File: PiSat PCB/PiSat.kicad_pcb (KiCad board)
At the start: 4 copper layers, 85 x 56 mm, 125 parts, among them IC1 PNT-SG3FS-TR, J1 Conn_01x05_Pin, J3 Conn_01x06_Pin, J4 Conn_01x03_Pin, J5 Conn_01x05_Pin, J6 Conn_01x05_Pin, Q7 AO3407A, SW1 MSK12C02, SW2 SKRPACE010, SW3 SKRPACE010, U1 BQ24075RGTR, U12 AP2112K-3.3, U4 DW03C_C41367942, U5 SMA-KWE_C7498154, U6 ESP32-C3-MINI-1U-N4, X1 X322512MSB4SI

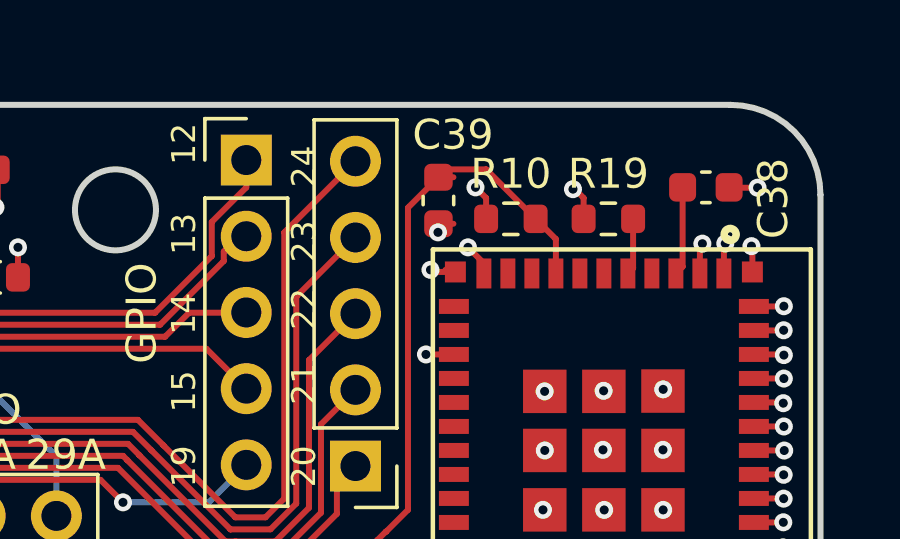
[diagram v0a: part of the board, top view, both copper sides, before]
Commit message: sync
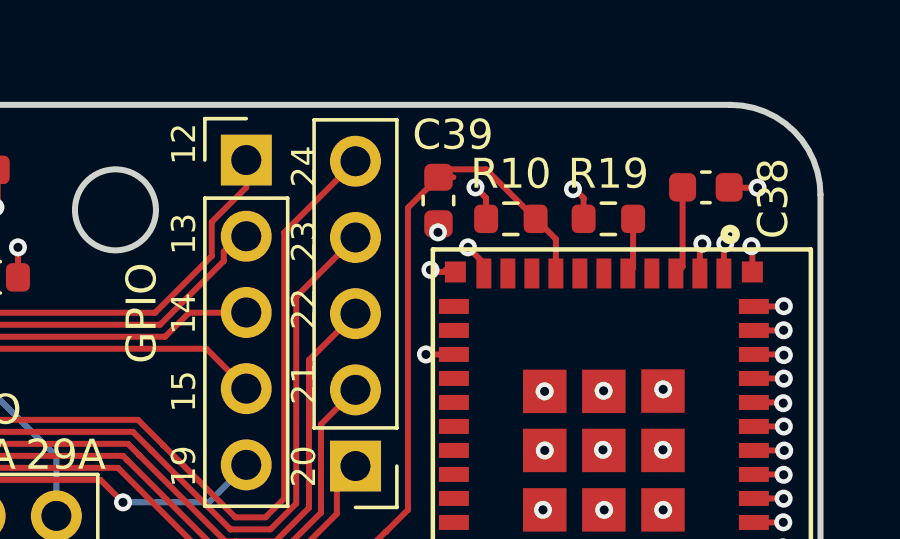
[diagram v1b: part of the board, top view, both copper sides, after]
